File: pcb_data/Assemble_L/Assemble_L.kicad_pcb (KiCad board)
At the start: 2 copper layers, 164.3 x 102.4 mm, 75 parts, among them U1 XIAO-nRF52840-DIP

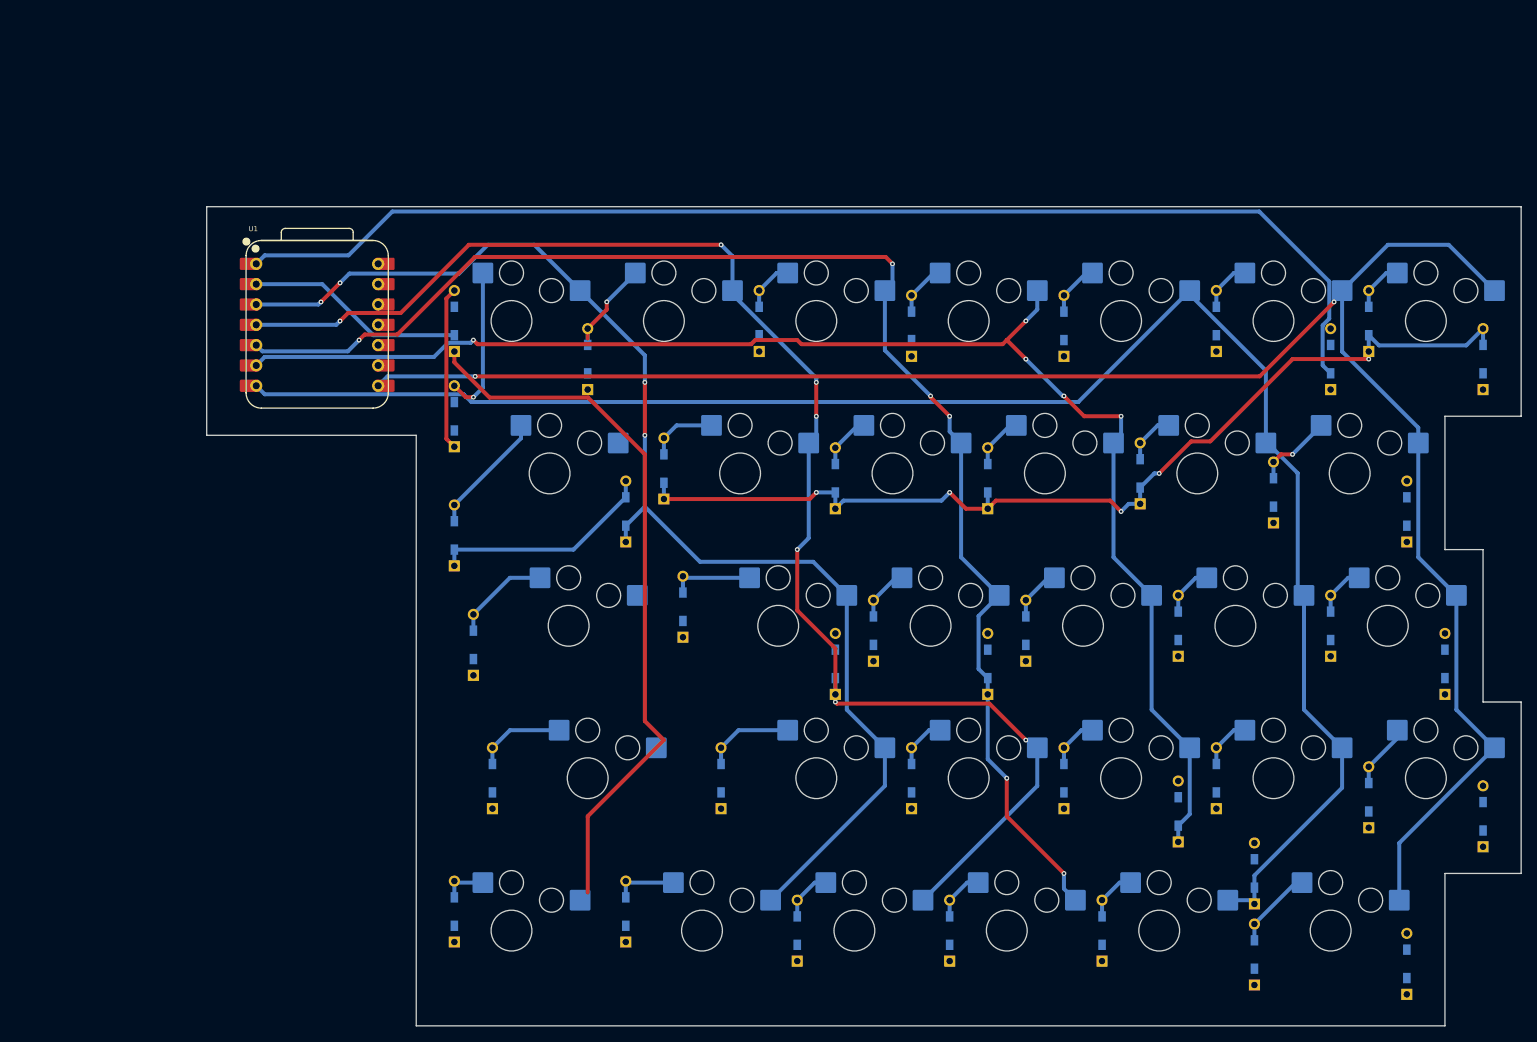
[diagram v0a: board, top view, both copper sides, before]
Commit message: update symbol
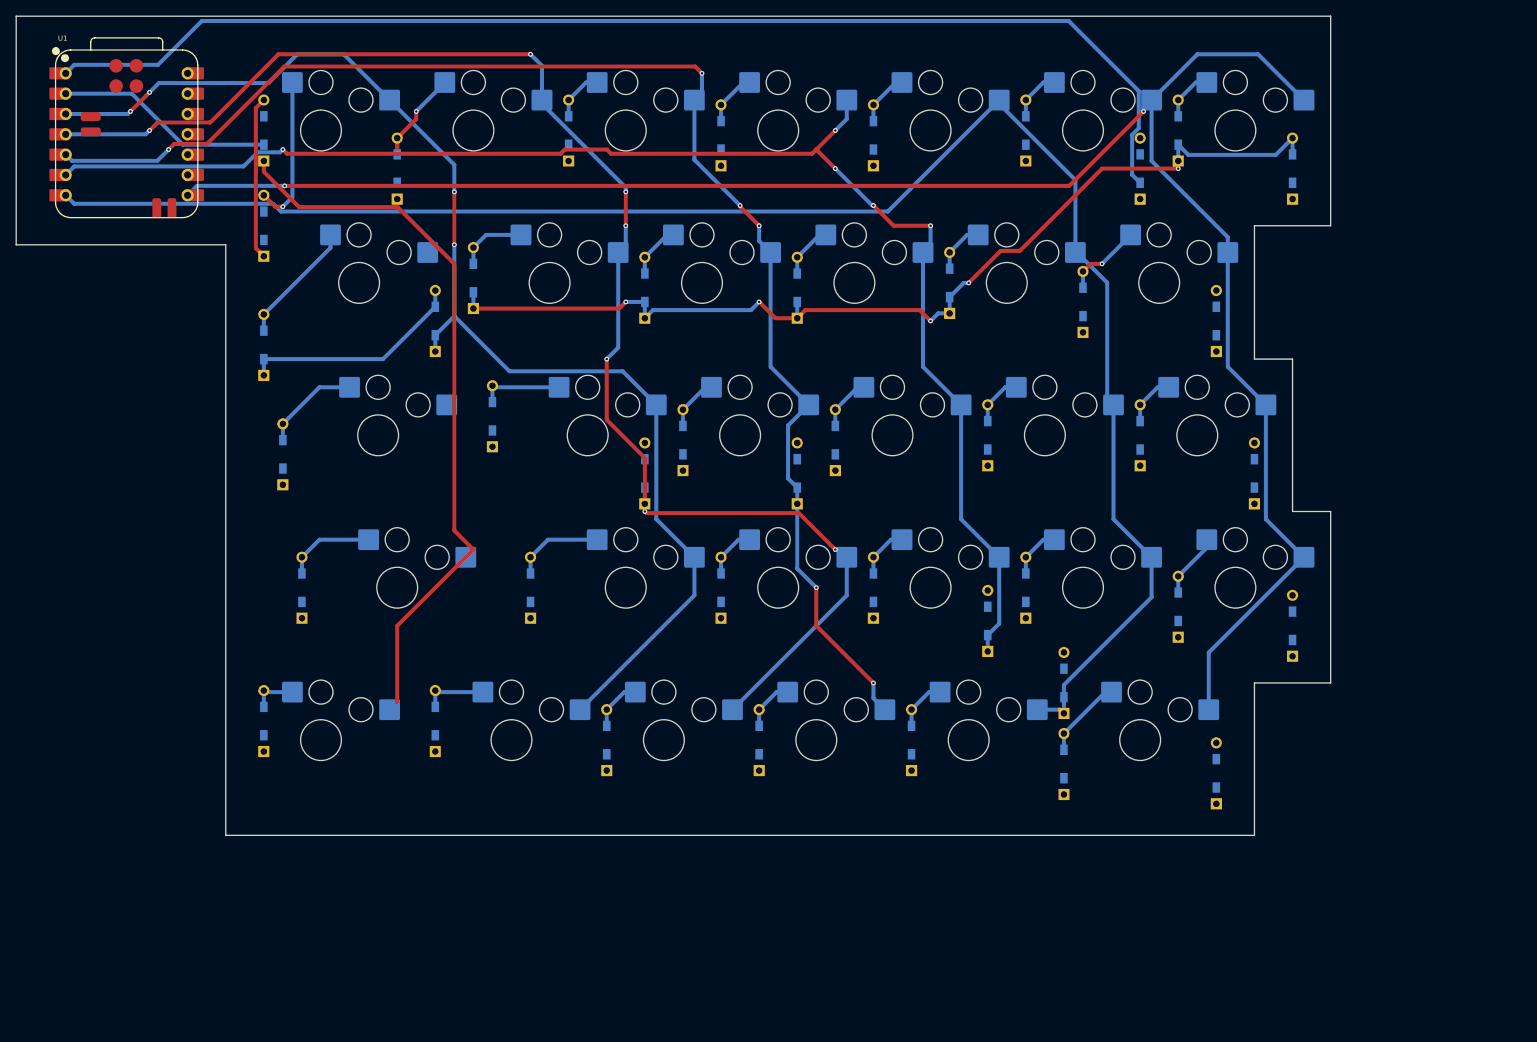
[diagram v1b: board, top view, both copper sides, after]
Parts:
- U1: value XIAO-nRF52840-DIP -> XIAO-nRF52840; footprint Seeed Studio XIAO Series Library:XIAO-nRF52840-DIP -> custom-library:XIAO-nRF52840
- moved D0-3 33.7 mm to (78.6, 114.3)
- moved D1-3 33.7 mm to (107.2, 114.3)
- moved D2-3 33.7 mm to (131.0, 114.3)
- moved D3-2 33.7 mm to (126.2, 95.9)
- moved D4-3 33.7 mm to (150.0, 114.3)
- moved D5-3 33.7 mm to (169.1, 114.3)
- moved D6-0 33.7 mm to (169.1, 57.1)
- moved D6-1 33.7 mm to (188.1, 57.1)
- moved DS0 33.7 mm to (73.8, 57.1)
- moved DS4 33.7 mm to (164.3, 118.5)
- moved DS5 33.7 mm to (173.8, 126.2)
- moved RC0-3 33.7 mm to (90.5, 114.3)
- moved RC1-0 33.7 mm to (81.0, 57.1)
- moved RC1-2 33.7 mm to (114.3, 95.2)
- moved RC1-3 33.7 mm to (119.1, 114.3)
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
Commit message: temp
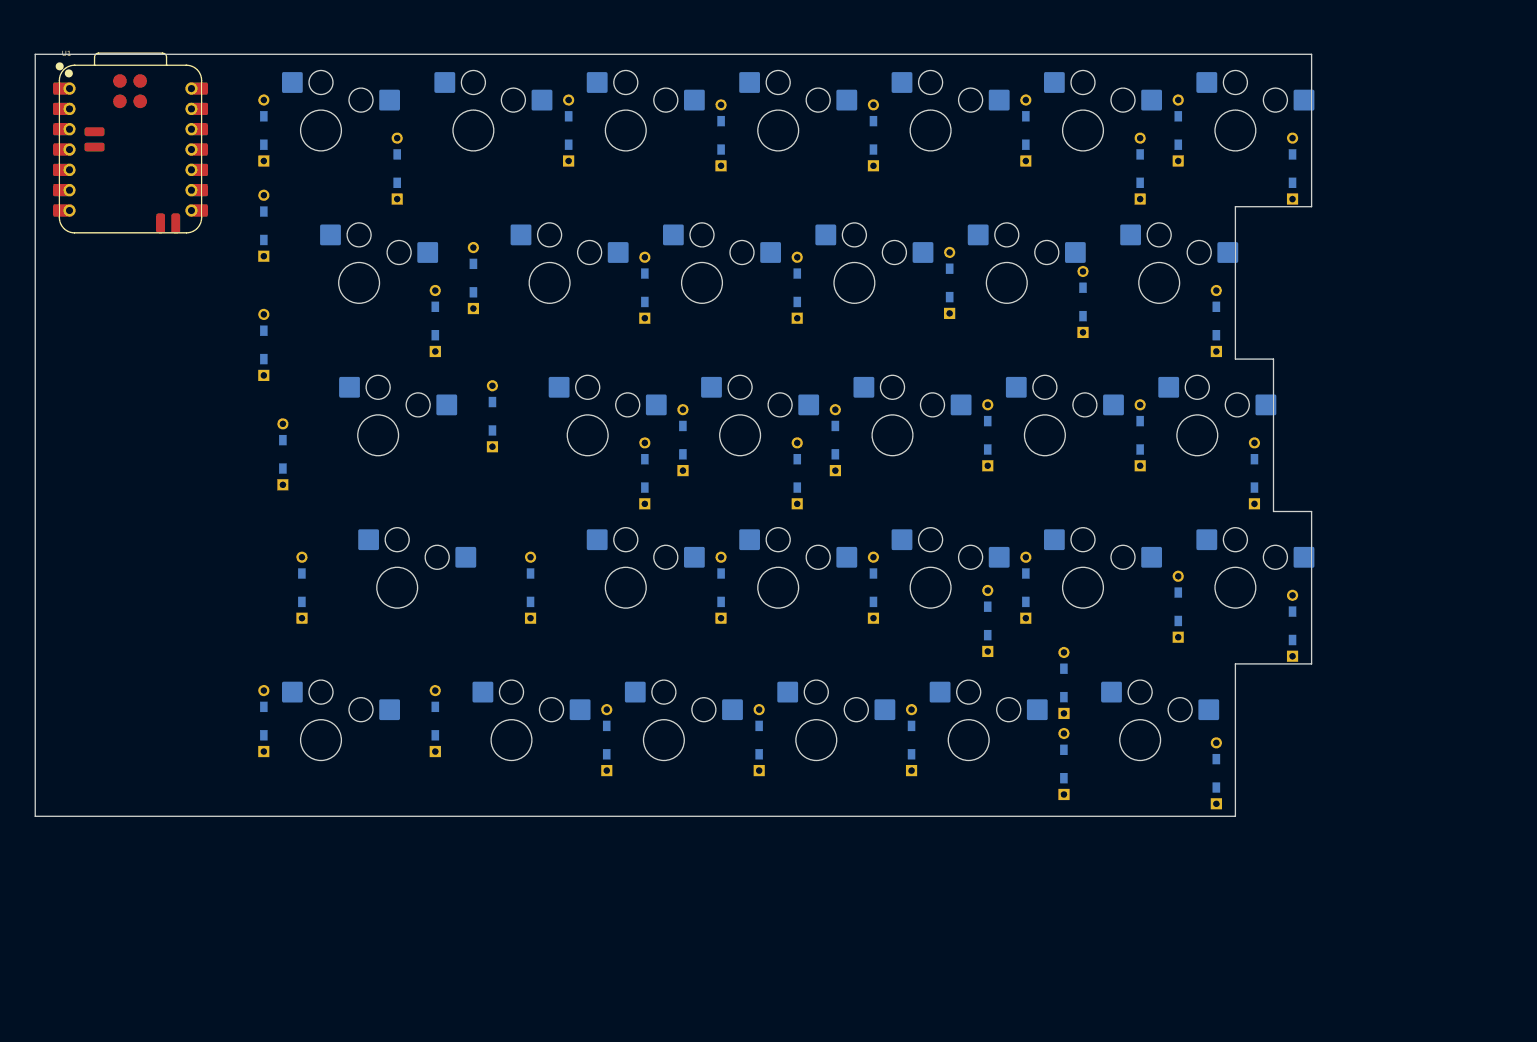
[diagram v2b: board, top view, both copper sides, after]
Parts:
- moved U1 1.96 mm to (57.1, 59.5)
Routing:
- net IO 6: track 238.5 -> 0.00 mm, vias 2 -> 0
- net IO 5: track 216.0 -> 0.00 mm
- net IO 4: track 180.1 -> 0.00 mm, vias 5 -> 0
- net IO 2: track 180.1 -> 0.00 mm, vias 7 -> 0
- net IO 3: track 177.0 -> 0.00 mm, vias 6 -> 0
- net IO 1: track 157.5 -> 0.00 mm, vias 4 -> 0
- net Net-(D0-1-K): track 155.2 -> 0.00 mm, vias 5 -> 0
- net INTR_L: track 152.7 -> 0.00 mm
- net IO 0: track 117.0 -> 0.00 mm
- net Net-(D1-0-K): track 20.4 -> 0.00 mm
- net Net-(D1-0-A): track 19.0 -> 0.00 mm, vias 1 -> 0
- net Net-(D0-1-A): track 15.4 -> 0.00 mm
- net Net-(D2-0-A): track 12.7 -> 0.00 mm, vias 1 -> 0
- net Net-(D0-2-A): track 12.3 -> 0.00 mm
- net Net-(D1-3-A): track 11.3 -> 0.00 mm
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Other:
- board size 164.3 x 102.4 mm -> 159.5 x 95.2 mm
